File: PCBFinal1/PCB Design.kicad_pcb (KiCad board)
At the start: 2 copper layers, 86 x 61.5 mm, 13 parts, among them J1 Screw_Terminal_01x02, J2 Screw_Terminal_01x03, J3 Screw_Terminal_01x03, J4 Screw_Terminal_01x02, J5 Screw_Terminal_01x02, K1 SANYOU_SRD_Form_C, Q1 BC547, U1 DEVKIT_V1_ESP32-WROOM-32

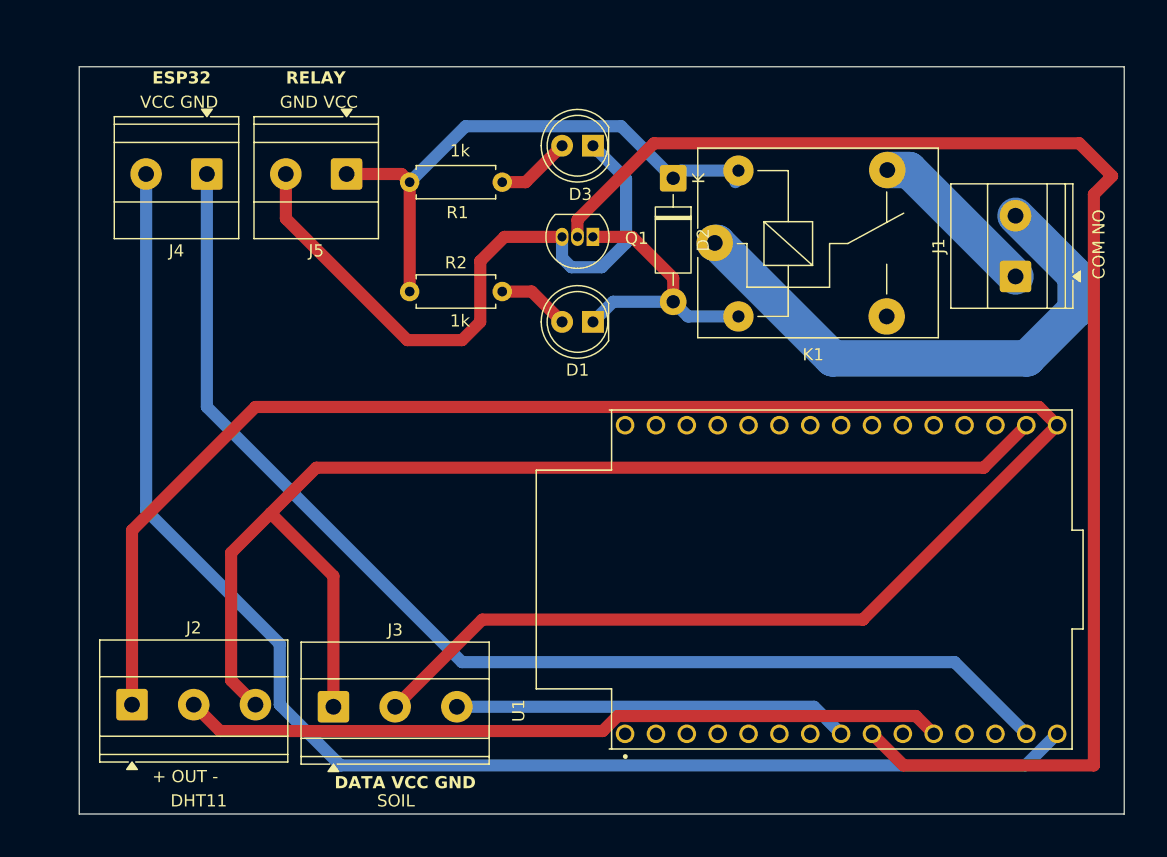
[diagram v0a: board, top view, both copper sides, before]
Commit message: Finished with the soil calibrations and first version of the pcb design.
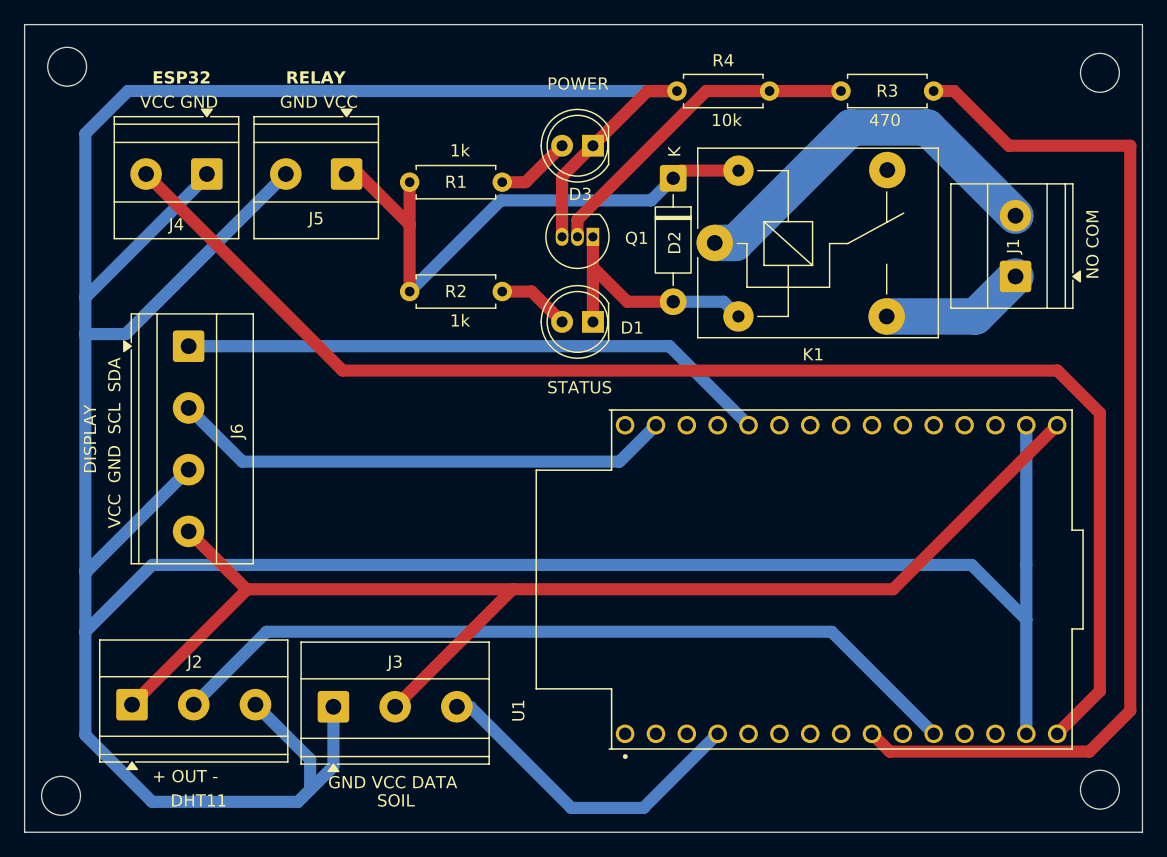
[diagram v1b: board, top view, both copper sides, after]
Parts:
- added J6: Screw_Terminal_01x04, TerminalBlock_Phoenix:TerminalBlock_Phoenix_MKDS-1,5-4-5.08_1x04_P5.08mm_Horizontal, F.Cu at (183.0, 63.0)
- added R3: 470, Resistor_THT:R_Axial_DIN0207_L6.3mm_D2.5mm_P7.62mm_Horizontal, F.Cu at (244.3, 42.0)
- added R4: 10k, Resistor_THT:R_Axial_DIN0207_L6.3mm_D2.5mm_P7.62mm_Horizontal, F.Cu at (223.2, 42.0)
- added REF**: MountingHole_3.2mm_M3_ISO14580, MountingHole:MountingHole_3.2mm_M3_ISO14580, F.Cu at (258.0, 40.5)
- added REF**: MountingHole_3.2mm_M3_ISO14580, MountingHole:MountingHole_3.2mm_M3_ISO14580, F.Cu at (258.0, 99.5)
- added REF**: MountingHole_3.2mm_M3_ISO14580, MountingHole:MountingHole_3.2mm_M3_ISO14580, F.Cu at (173.0, 40.0)
- added REF**: MountingHole_3.2mm_M3_ISO14580, MountingHole:MountingHole_3.2mm_M3_ISO14580, F.Cu at (172.5, 100.0)
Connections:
- J2 pad 3: Net-(J2-Pin_3) -> GND
- J3 pad 1: Net-(J2-Pin_3) -> GND
- J4 pad 1: Net-(J4-Pin_1) -> GND
- K1 pad 3: unconnected-(K1-Pad3) -> Net-(J1-Pin_1)
- K1 pad 4: Net-(J1-Pin_1) -> unconnected-(K1-Pad4)
- U1 pad 12: Net-(J3-Pin_3) -> unconnected-(U1-D12-Pad12)
- U1 pad 13: Net-(Q1-B) -> Net-(U1-D13)
- U1 pad 18: Net-(J4-Pin_1) -> GND
- U1 pad 21: Net-(J2-Pin_3) -> Net-(J6-Pin_1)
- U1 pad 22: unconnected-(U1-D22-Pad22) -> Net-(J6-Pin_2)
- U1 pad 34: unconnected-(U1-D34-Pad34) -> Net-(J3-Pin_3)
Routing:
- net GND: track 54.3 -> 309.9 mm
- net Net-(J2-Pin_3): track 101.2 -> 0.00 mm
- net Net-(J4-Pin_1): track 97.8 -> 0.00 mm
- net Net-(Q1-B): track 117.6 -> 27.5 mm
- net Net-(U1-D13): track 0.00 -> 87.8 mm
- net Net-(J2-Pin_1): track 159.4 -> 106.2 mm
- net Net-(J6-Pin_1): track 0.00 -> 48.8 mm
- net Net-(J6-Pin_2): track 0.00 -> 41.5 mm
- net Net-(J1-Pin_2): track 45.1 -> 31.7 mm
- net Net-(J3-Pin_3): track 32.5 -> 27.4 mm
- net Net-(J2-Pin_2): track 62.9 -> 66.9 mm
- net Net-(D1-K): track 23.1 -> 20.7 mm
- net Net-(J1-Pin_1): track 14.2 -> 12.0 mm
- net Net-(D2-K): track 46.5 -> 48.7 mm
- net Net-(J4-Pin_2): track 115.4 -> 114.5 mm
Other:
- board size 86 x 61.5 mm -> 92 x 66.5 mm
- board text added: "10k"
- board text added: "470"
- board text added: "DISPLAY"
- board text added: "GND VCC DATA"
- board text added: "NO COM"
- board text added: "POWER"
- board text added: "STATUS"
- board text added: "VCC GND SCL SDA"
- board text removed: "COM NO"
- board text removed: "DATA VCC GND"
